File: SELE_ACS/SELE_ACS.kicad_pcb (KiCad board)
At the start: 2 copper layers, 20 parts, among them J1 AVR-ISP-6, J2 Input Cables, J3 FT232 Adapter, SW1 Button Reset, SW2 SW_DIP_x04, U1 atmega328p, U2 MAX485E, U3 LM7805_TO220, Y1 Crystal 8MHz

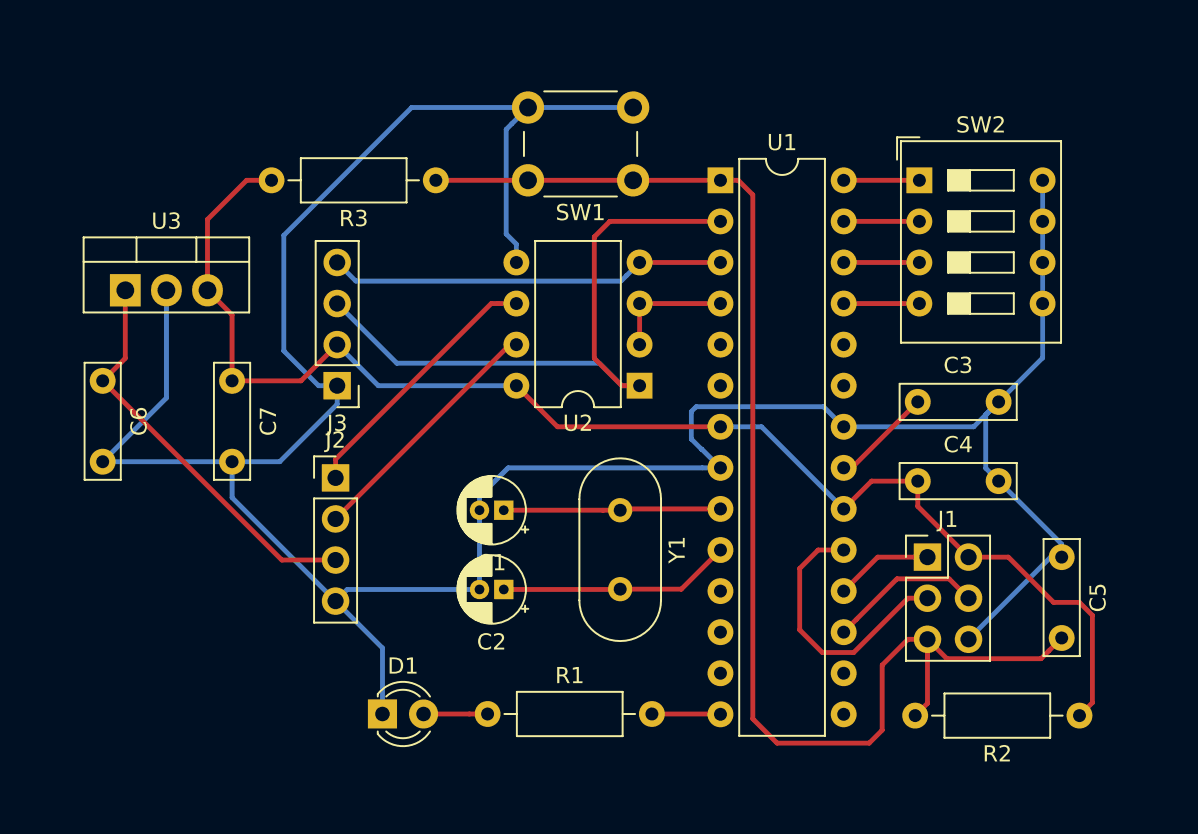
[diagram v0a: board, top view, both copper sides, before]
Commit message: Add files via upload
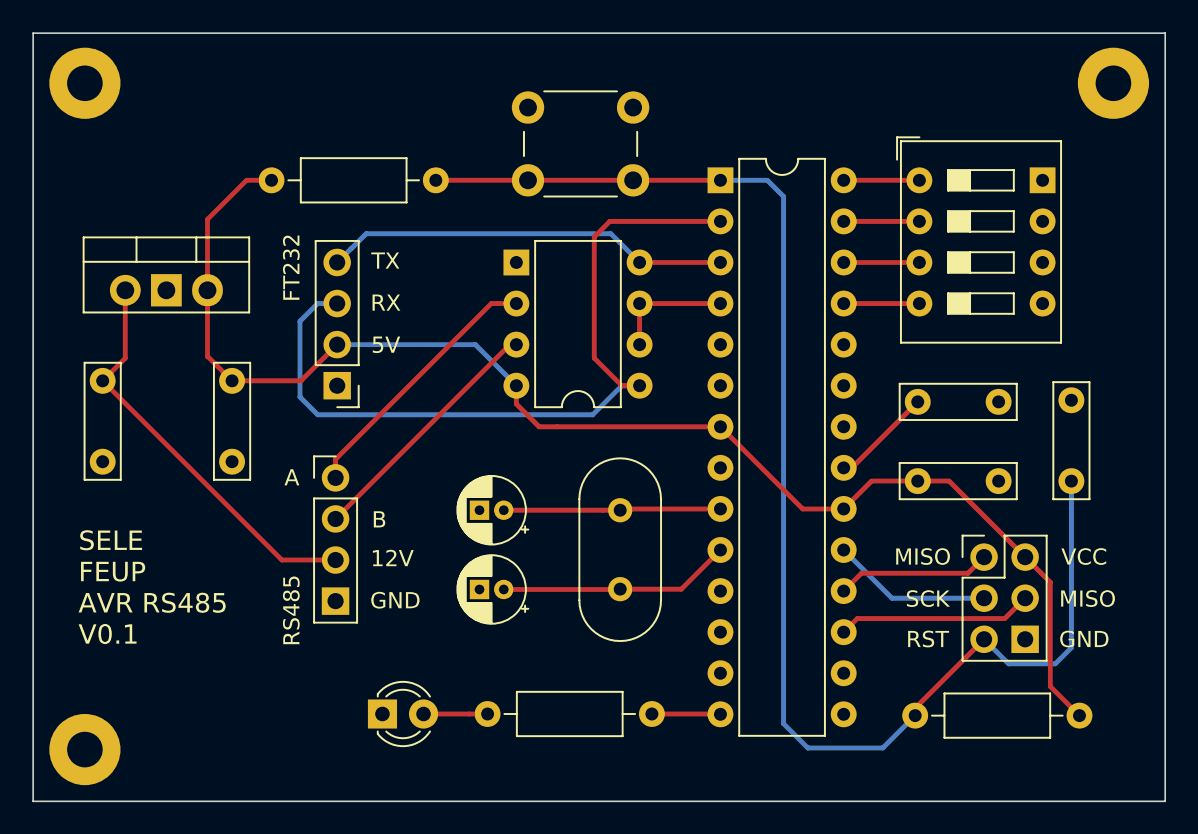
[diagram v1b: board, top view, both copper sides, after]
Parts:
- added REF**: MountingHole_2.2mm_M2_Pad, MountingHole:MountingHole_2.2mm_M2_Pad, F.Cu at (80.6, 107.8)
- added REF**: MountingHole_2.2mm_M2_Pad, MountingHole:MountingHole_2.2mm_M2_Pad, F.Cu at (80.6, 66.6)
- added REF**: MountingHole_2.2mm_M2_Pad, MountingHole:MountingHole_2.2mm_M2_Pad, F.Cu at (144.2, 66.6)
- moved C5 9.72 mm to (141.6, 86.2)
- moved J1 3.50 mm to (136.2, 95.9)
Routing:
- net GND: track 185.1 -> 0.00 mm
- net RX: track 40.0 -> 48.8 mm
- net SCK: track 16.9 -> 9.91 mm
- net MISO: track 6.05 -> 9.55 mm
- net RESET: track 84.4 -> 87.3 mm
- net MOSI: track 9.58 -> 12.1 mm
- net AVCC: track 85.7 -> 84.5 mm
- net TX: track 24.7 -> 25.2 mm
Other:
- board outline added: 70 x 47.5 mm
- board text added: "12V"
- board text added: "5V"
- board text added: "A"
- board text added: "B"
- board text added: "FT232"
- board text added: "GND"
- board text added: "MISO"
- board text added: "RS485"
- board text added: "RST"
- board text added: "RX"
- board text added: "SCK"
- board text added: "SELE FEUP AVR RS485 V0.1"
- board text added: "TX"
- board text added: "VCC"
